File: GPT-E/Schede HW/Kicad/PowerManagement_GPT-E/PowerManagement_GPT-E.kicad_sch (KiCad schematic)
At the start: 67 parts, among them J1 Battery, J2 switch, J3 Conn_01x02_Socket, J4 Conn_02x02_Counter_Clockwise, J5 Conn_01x02, J6 Conn_01x02, J7 Charge_conn, J8 Voltage_indicator, J9 Buzzer_Accensione, Q1 IRLZ44N, Q2 IRF7416TRPBF, SW1 SW_SPDT, U1 ATmega8-16P, U2 BMS_3S_LithiumBattery18650, U3 NRF24L01_Breakout, U4 LM393, U5 MP1584, Y1 16MHz

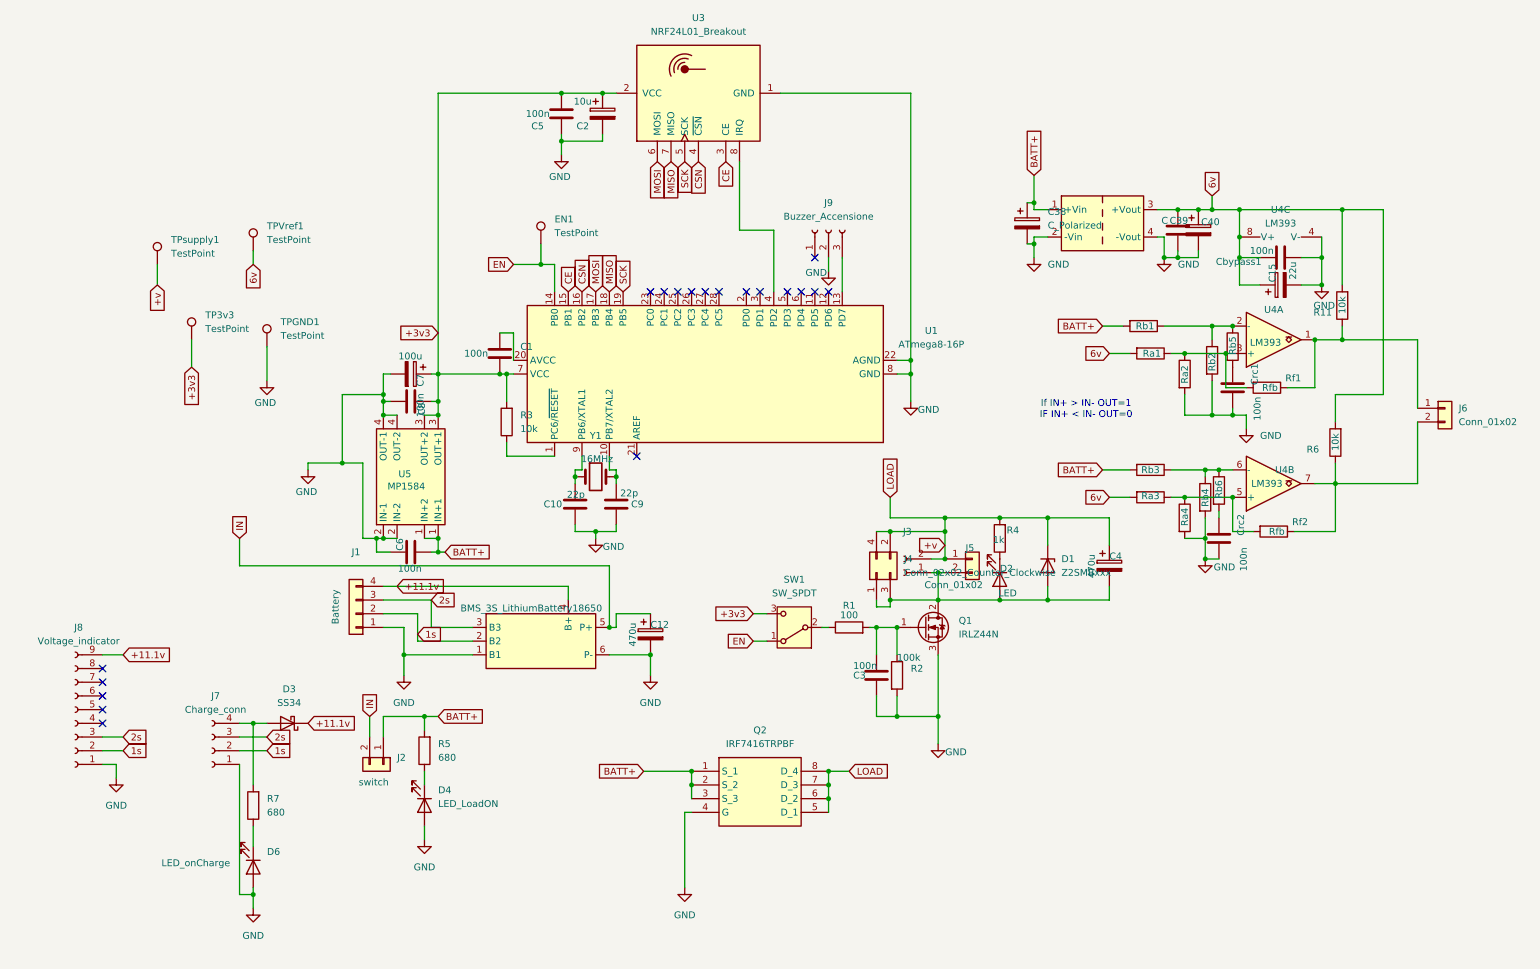
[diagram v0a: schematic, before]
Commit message: up
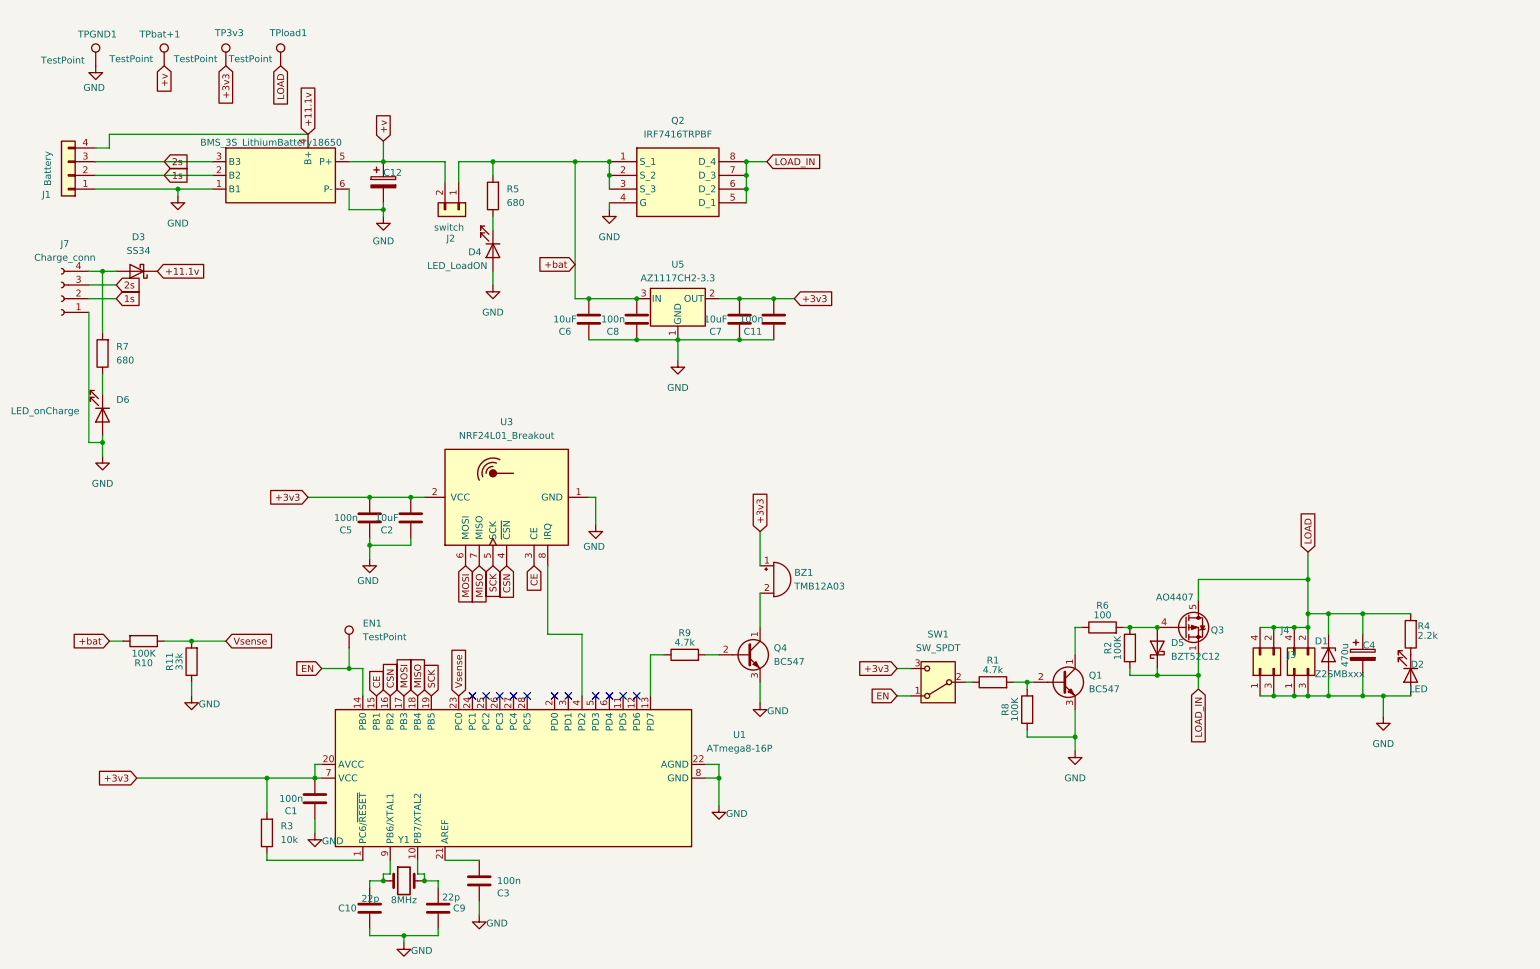
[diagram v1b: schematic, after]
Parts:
- removed C15: 22u, Capacitor_THT:CP_Radial_D6.3mm_P2.50mm, symbol Device:C_Polarized
- removed C2: 10u, Capacitor_THT:CP_Radial_D8.0mm_P3.50mm, symbol Device:C_Polarized
- removed C38, C40: C_Polarized, Capacitor_THT:CP_Radial_D6.3mm_P2.50mm, symbol Device:C_Polarized
- removed C39: C, Capacitor_THT:C_Disc_D5.1mm_W3.2mm_P5.00mm, symbol Device:C
- removed C7: 100u, Capacitor_THT:CP_Radial_D8.0mm_P3.50mm, symbol Device:C_Polarized
- removed Cbypass1, Crc1, Crc2: 100n, Capacitor_THT:C_Disc_D5.1mm_W3.2mm_P5.00mm, symbol Device:C
- removed J3: Conn_01x02_Socket, Connector_PinSocket_2.54mm:PinSocket_1x02_P2.54mm_Vertical, symbol Connector:Conn_01x02_Socket
- removed J5, J6: Conn_01x02, Connector_Molex:Molex_KK-254_AE-6410-02A_1x02_P2.54mm_Vertical, symbol Connector_Generic:Conn_01x02
- removed J8: Voltage_indicator, Connector_PinHeader_2.54mm:PinHeader_1x09_P2.54mm_Vertical, symbol Connector:Conn_01x09_Socket
- removed J9: Buzzer_Accensione, Connector:FanPinHeader_1x03_P2.54mm_Vertical, symbol Connector:Conn_01x03_Socket
- removed Q1: IRLZ44N, Package_TO_SOT_THT:TO-220-3_Horizontal_TabDown, symbol Transistor_FET:IRLZ44N
- removed Ra1, Ra3, Rb5, Rb6: 22k, Resistor_THT:R_Axial_DIN0204_L3.6mm_D1.6mm_P5.08mm_Horizontal, symbol Device:R
- removed Ra2, Ra4, Rb2, Rb4: 10k, Resistor_THT:R_Axial_DIN0204_L3.6mm_D1.6mm_P5.08mm_Horizontal, symbol Device:R
- removed Rb1, Rb3: 47k, Resistor_THT:R_Axial_DIN0204_L3.6mm_D1.6mm_P5.08mm_Horizontal, symbol Device:R
- removed Rf1, Rf2: Rfb, Resistor_THT:R_Axial_DIN0204_L3.6mm_D1.6mm_P5.08mm_Horizontal, symbol Device:R
- removed TPVref1: TestPoint, TestPoint:TestPoint_Pad_2.0x2.0mm, symbol Connector:TestPoint
- removed U4: LM393, Package_DIP:DIP-8_W7.62mm, symbol Comparator:LM393
- removed U5: MP1584, Converter_DCDC:MP1584, symbol Personale:MP1584
- removed U8: ~, LIB_Personale:Mini360, symbol Libreria_Personale:Mini360_DCDC_stepdown
- added BZ1: TMB12A03, Buzzer_Beeper:Buzzer_12x9.5RM7.6, symbol Device:Buzzer
- added C11: 100n, Capacitor_SMD:C_0805_2012Metric_Pad1.18x1.45mm_HandSolder, symbol Device:C
- added C2, C7: 10uF, Capacitor_SMD:C_0805_2012Metric_Pad1.18x1.45mm_HandSolder, symbol Device:C
- added D5: BZT52C12, Diode_SMD:D_SOD-123, symbol Diode:BAT48ZFILM
- added J3: Conn_02x02_Counter_Clockwise, Connector_Molex:Molex_Micro-Fit_3.0_43045-0412_2x02_P3.00mm_Vertical, symbol Connector_Generic:Conn_02x02_Counter_Clockwise
- added Q1, Q4: BC547, Package_TO_SOT_THT:TO-92L_Inline, symbol Transistor_BJT:BC547
- added Q3: AO4407, Package_SO:SOIC-8_3.9x4.9mm_P1.27mm, symbol Transistor_FET:FDS9435A
- added R10: 100K, Resistor_THT:R_Axial_DIN0204_L3.6mm_D1.6mm_P5.08mm_Horizontal, symbol Device:R
- added R8: 100K, Resistor_SMD:R_1206_3216Metric_Pad1.30x1.75mm_HandSolder, symbol Device:R
- added R9: 4.7k, Resistor_SMD:R_1206_3216Metric_Pad1.30x1.75mm_HandSolder, symbol Device:R
- added TPload1: TestPoint, TestPoint:TestPoint_Pad_2.0x2.0mm, symbol Connector:TestPoint
- added U5: AZ1117CH2-3.3, Package_TO_SOT_SMD:SOT-223-3_TabPin2, symbol Regulator_Linear:AZ1117CH2-3.3
- C1, C10, C3, C5, C8, C9: footprint Capacitor_THT:C_Disc_D7.0mm_W2.5mm_P5.00mm -> Capacitor_SMD:C_0805_2012Metric_Pad1.18x1.45mm_HandSolder
- C6: value 100n -> 10uF; footprint Capacitor_THT:C_Disc_D7.0mm_W2.5mm_P5.00mm -> Capacitor_SMD:C_0805_2012Metric_Pad1.18x1.45mm_HandSolder
- R1: value 100 -> 4.7k; footprint Resistor_THT:R_Axial_DIN0204_L3.6mm_D1.6mm_P5.08mm_Horizontal -> Resistor_SMD:R_1206_3216Metric_Pad1.30x1.75mm_HandSolder
- R11: value 10k -> 33k
- R2: value 100k -> 100K; footprint Resistor_THT:R_Axial_DIN0204_L3.6mm_D1.6mm_P5.08mm_Horizontal -> Resistor_SMD:R_1206_3216Metric_Pad1.30x1.75mm_HandSolder
- R4: value 1k -> 2.2k
- R6: value 10k -> 100; footprint Resistor_THT:R_Axial_DIN0204_L3.6mm_D1.6mm_P5.08mm_Horizontal -> Resistor_SMD:R_1206_3216Metric_Pad1.30x1.75mm_HandSolder
- Y1: value 16MHz -> 8MHz
- renumbered TPsupply1 to TPbat+1
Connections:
- net IN is gone; now on net +v: C12.1, J2.2 (Pin_2), U2.5 (P+)
- net +3v3: now also C1.1, U1.20 (AVCC), BZ1.1 (+), C11.1, C2.1, C7.1, U5.2 (OUT); no longer C1.2, C8.1
- net +v: no longer C4.1, D1.1 (K), J4.2 (Pin_2), J4.4 (Pin_4), Q2.5 (D_1), Q2.6 (D_2), Q2.7 (D_3), Q2.8 (D_4), R4.2
- net GND: now also C1.2, C4.2, C6.2, D1.2 (A), D2.2 (A), J4.1 (Pin_1), J4.3 (Pin_3), R11.1, C11.2, C2.2, C7.2, J3.1 (Pin_1), J3.3 (Pin_3), Q1.3 (E), Q4.3 (E), R8.1, U5.1 (GND); no longer C6.1, R2.2
- net at R6.1: now also Q1.1 (C)
- net at U1.13 (PD7): now also R9.1
- net at U1.21 (AREF): now also C3.1
- net Vsense: now reaches U1.23 (PC0)
- net Vsense: now also R11.2, R10.1
- net 6v: no longer names the net of R6.2
- net 6v: now also R2.2, D5.2 (A), Q3.4 (G); no longer R11.2
- net BATT+ renamed +bat
- net +bat: now also C6.1, C8.1, R10.2, U5.3 (IN); no longer C6.2
- new net: Q4.2 (B), R9.2
- new net: Q1.2 (B), R1.2, R8.2
- new net: BZ1.2 (-), Q4.1 (C)
- new net LOAD: C4.1, D1.1 (K), J3.2 (Pin_2), J3.4 (Pin_4), J4.2 (Pin_2), J4.4 (Pin_4), Q3.5 (D), Q3.6 (D), Q3.7 (D), Q3.8 (D), R4.2, TPload1.1
- new net LOAD_IN: D5.1 (K), Q2.5 (D_1), Q2.6 (D_2), Q2.7 (D_3), Q2.8 (D_4), Q3.1 (S), Q3.2 (S), Q3.3 (S), R2.1
- no-connect marks 19 -> 11
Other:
- note removed: "If IN+ > IN- OUT=1 IF IN+ < IN- OUT=0"
- moved on the sheet: C10, C12, C4, C5, C9, D1, D2, D3, D4, D6, EN1, J1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
